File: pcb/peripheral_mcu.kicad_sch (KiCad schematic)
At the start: 4 parts, among them U4 STM32C071RBTx

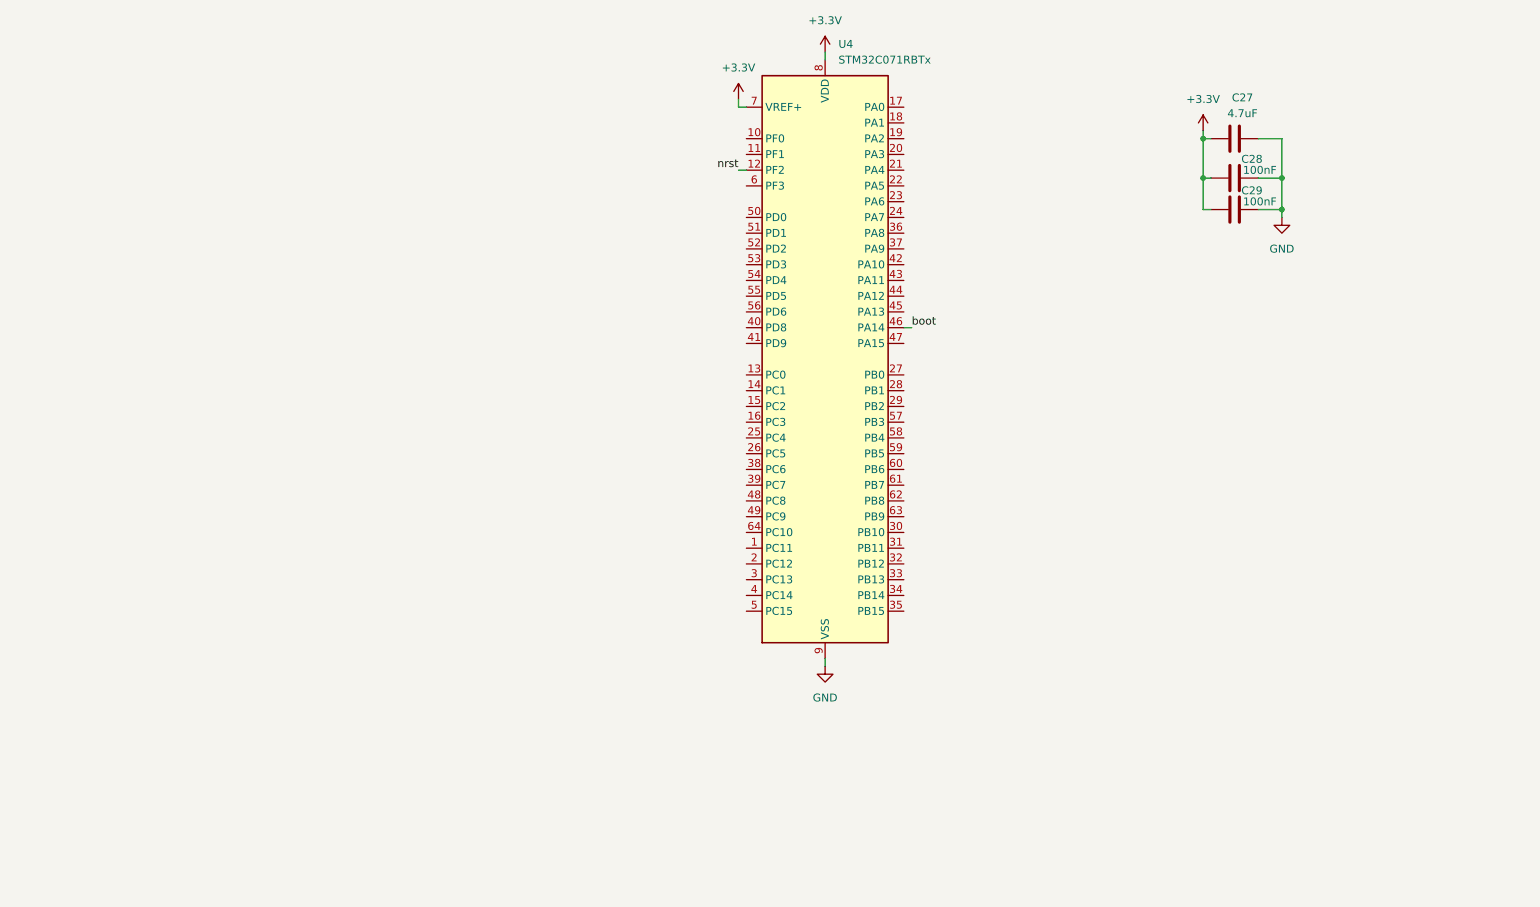
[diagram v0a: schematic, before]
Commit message: tons of work on rf and mcu
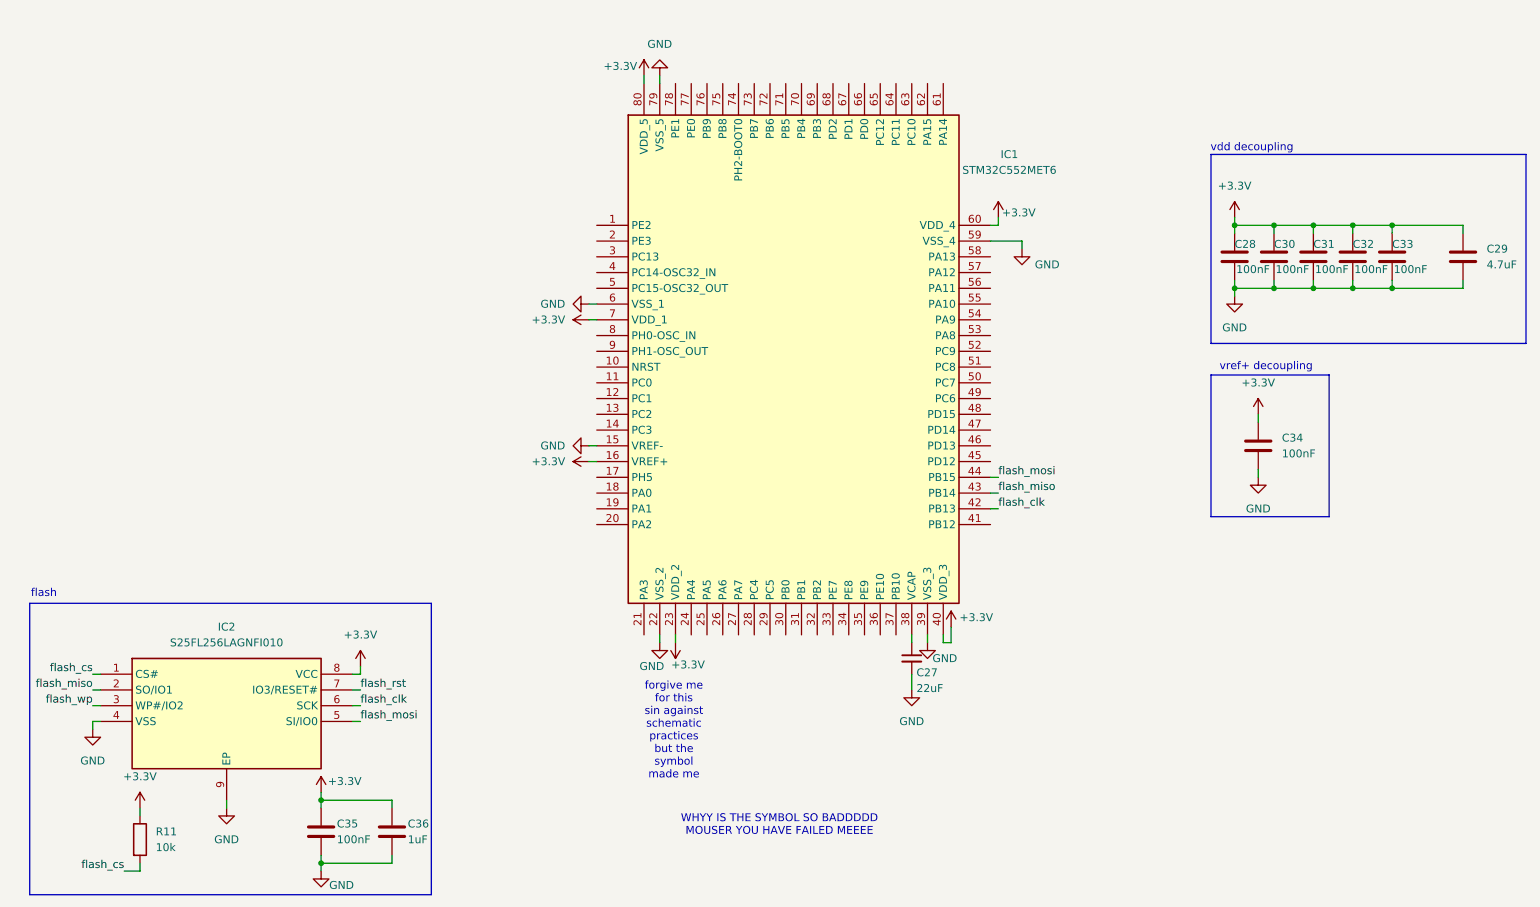
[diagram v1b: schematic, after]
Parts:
- removed C27: 4.7uF, symbol Device:C
- removed U4: STM32C071RBTx, Package_QFP:LQFP-64_10x10mm_P0.5mm, symbol MCU_ST_STM32C0:STM32C071RBTx
- added C27: 22uF, symbol Device:C_Small
- added C30, C31, C32, C33, C34, C35: 100nF, symbol Device:C
- added C36: 1uF, symbol Device:C
- added IC1: STM32C552MET6, QFP50P1400X1400X160-80N, symbol STM32C552MET6:STM32C552MET6
- added IC2: S25FL256LAGNFI010, SON127P800X600X80-9N-D, symbol S25FL256LAGNFI010:S25FL256LAGNFI010
- added R11: 10k, symbol Device:R
- C29: value 100nF -> 4.7uF
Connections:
- net +3.3V: now also C30.1, C31.1, C32.1, C33.1, C34.1, C35.1, C36.1, IC1.16 (VREF+), IC1.23 (VDD_2), IC1.40 (VDD_3), IC1.60 (VDD_4), IC1.7 (VDD_1), IC1.80 (VDD_5), IC2.8 (VCC), R11.1
- net GND: now also C27.2, C30.2, C31.2, C32.2, C33.2, C34.2, C35.2, C36.2, IC1.15 (VREF-), IC1.22 (VSS_2), IC1.39 (VSS_3), IC1.59 (VSS_4), IC1.6 (VSS_1), IC1.79 (VSS_5), IC2.4 (VSS), IC2.9 (EP)
- new net: C27.1, IC1.38 (VCAP)
- new net flash_clk: IC1.42 (PB13), IC2.6 (SCK)
- new net flash_cs: IC2.1 (CS#), R11.2
- new net flash_miso: IC1.43 (PB14), IC2.2 (SO/IO1)
- new net flash_mosi: IC1.44 (PB15), IC2.5 (SI/IO0)
- new net flash_rst: IC2.7 (IO3/RESET#)
- new net flash_wp: IC2.3 (WP#/IO2)
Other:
- note added: "WHYY IS THE SYMBOL SO BADDDDD MOUSER YOU HAVE FAILED MEEEE"
- note added: "flash"
- note added: "forgive me for this sin against schematic practices but the symbol made me"
- note added: "vdd decoupling"
- note added: "vref+ decoupling"

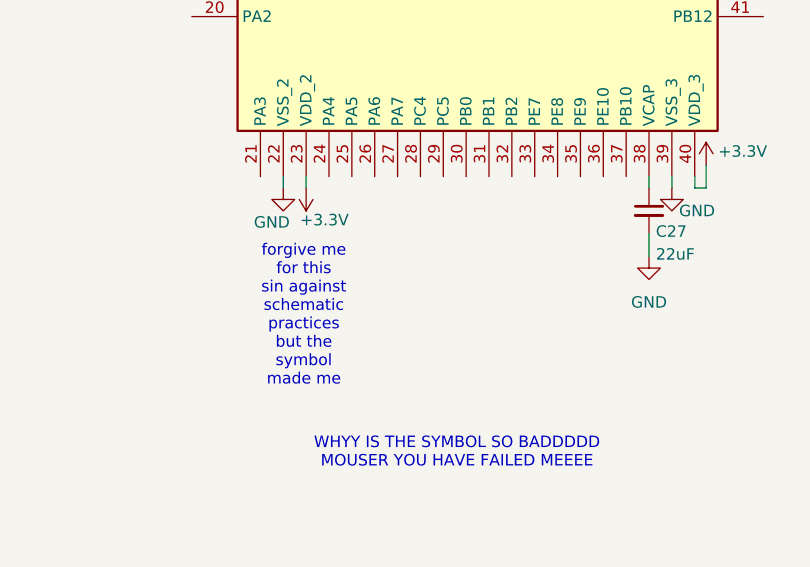
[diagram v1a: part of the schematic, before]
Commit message: added missing files, rf stuff done I think (hope)
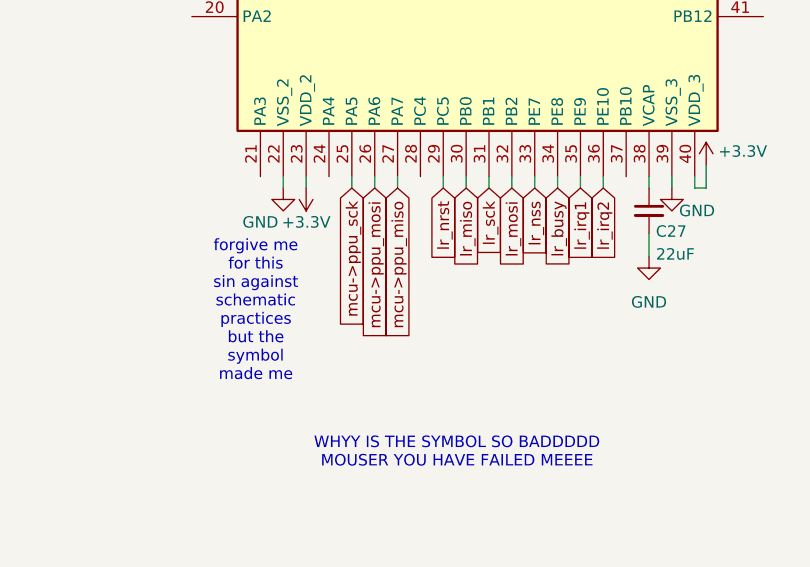
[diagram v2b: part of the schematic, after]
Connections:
- net mcu->ppu_sck: now reaches IC1.25 (PA5)
- net mcu->ppu_mosi: now reaches IC1.26 (PA6)
- net mcu->ppu_miso: now reaches IC1.27 (PA7)
- net lr_nrst: now reaches IC1.29 (PC5)
- net lr_miso: now reaches IC1.30 (PB0)
- net lr_sck: now reaches IC1.31 (PB1)
- net lr_mosi: now reaches IC1.32 (PB2)
- net lr_nss: now reaches IC1.33 (PE7)
- net lr_busy: now reaches IC1.34 (PE8)
- net lr_irq1: now reaches IC1.35 (PE9)
- net lr_irq2: now reaches IC1.36 (PE10)
